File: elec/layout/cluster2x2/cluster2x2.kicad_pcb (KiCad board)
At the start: 2 copper layers, 20 parts

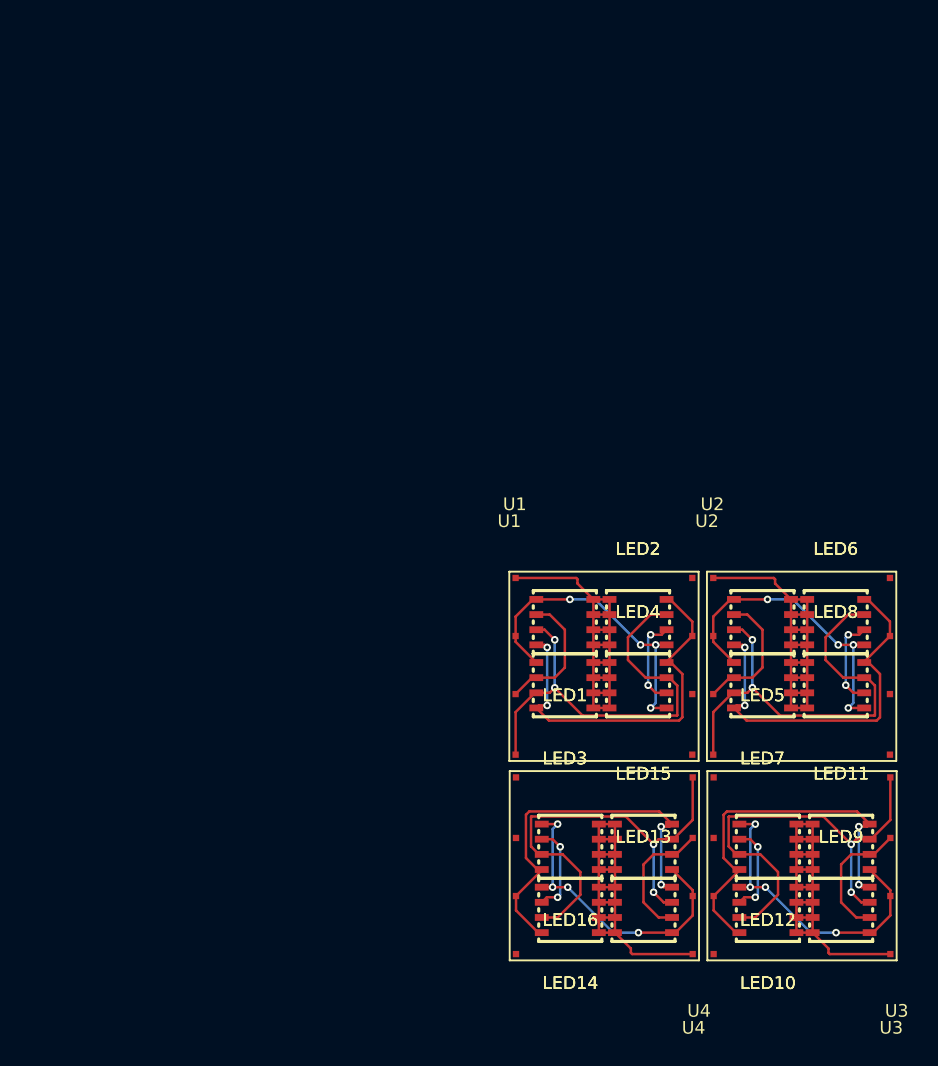
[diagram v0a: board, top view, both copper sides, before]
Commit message: cluster with driver
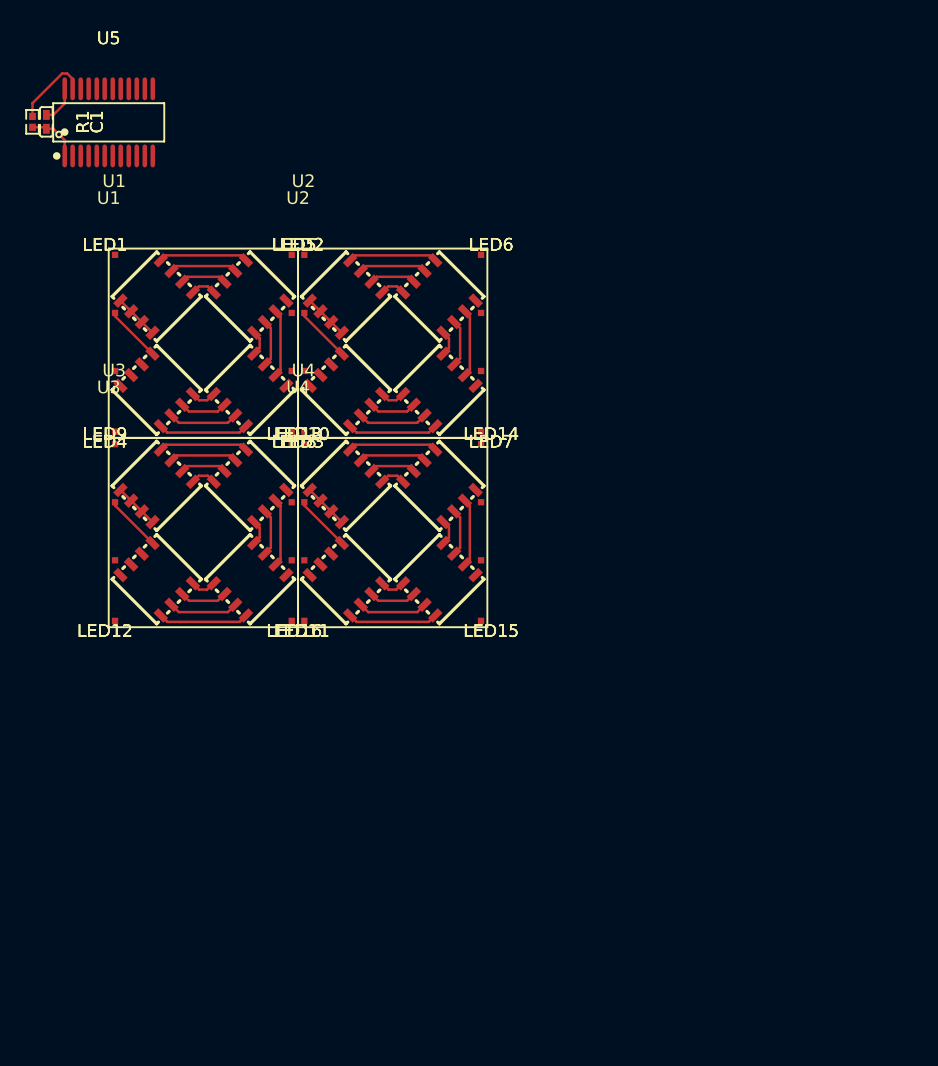
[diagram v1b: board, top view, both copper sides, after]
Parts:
- added C1: 100nF ±10% 16V X7R, Samsung_Electro_Mechanics_CL05B104KO5NNNC:C0402, F.Cu at (-4.94, -10.0)
- added R1: 309Ω ±1% 62.5mW, VO_SCR0402F309R:R0402, F.Cu at (-6.04, -10.0)
- added U5: , MBI_MBI5043GP_A:SSOP-24_L8.8-W4.0-P0.64-LS6.2-BL, F.Cu at (0.00, -10.0)
- moved U3 74.9 mm to (0.00, 15.0), turned to 0 degrees
- moved LED9 63.8 mm to (3.80, 18.8), turned to 45 degrees
- moved LED10 53.0 mm to (11.2, 18.8), turned to -45 degrees
- moved LED12 52.9 mm to (3.80, 26.2), turned to 135 degrees
- moved U4 52.2 mm to (15.0, 15.0), turned to 0 degrees
- moved LED11 51.4 mm to (11.2, 26.2), turned to -135 degrees
- moved LED8 45.3 mm to (18.8, 11.2), turned to 135 degrees
- moved LED4 44.7 mm to (3.80, 11.2), turned to 135 degrees
- moved LED5 41.9 mm to (18.8, 3.80), turned to 45 degrees
- moved LED1 41.4 mm to (3.80, 3.80), turned to 45 degrees
- moved U2 41.3 mm to (15.0, 0.00)
- moved LED13 41.0 mm to (18.8, 18.8), turned to 45 degrees
- moved U1 40.8 mm to (0.00, 0.00)
- moved LED6 40.6 mm to (26.2, 3.80), turned to -45 degrees
- moved LED2 40.1 mm to (11.2, 3.80), turned to -45 degrees
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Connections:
- net rows[0].pixels[0]-cathode_ir renamed rows[0].pixels[0]-ir
- net rows[0].pixels[0]-cathode_uv renamed rows[0].pixels[0]-uv
- net rows[0].pixels[0]-cathode_warm_white renamed rows[0].pixels[0]-warm_white
- net rows[0].pixels[1]-cathode_ir renamed rows[0].pixels[1]-ir
- net rows[0].pixels[1]-cathode_uv renamed rows[0].pixels[1]-uv
- net rows[0].pixels[1]-cathode_warm_white renamed rows[0].pixels[1]-warm_white
- net rows[1].pixels[0]-cathode_ir renamed rows[1].pixels[0]-ir
- net rows[1].pixels[0]-cathode_uv renamed rows[1].pixels[0]-uv
- net rows[1].pixels[0]-cathode_warm_white renamed rows[1].pixels[0]-warm_white
- net rows[1].pixels[1]-cathode_ir renamed rows[1].pixels[1]-ir
- net rows[1].pixels[1]-cathode_uv renamed rows[1].pixels[1]-uv
- net rows[1].pixels[1]-cathode_warm_white renamed rows[1].pixels[1]-warm_white
- LED1 pad 1: rows[0].pixels[0]-cathode_cold_white -> rows[0].pixels[0]-cold_white-1
- LED1 pad 2: rows[0].pixels[0]-anode -> -anode
- LED1 pad 3: rows[0].pixels[0]-cathode_blue -> rows[0].pixels[0]-blue-1
- LED1 pad 4: rows[0].pixels[0]-anode -> -anode
- LED1 pad 5: rows[0].pixels[0]-cathode_green -> rows[0].pixels[0]-green-1
- LED1 pad 6: rows[0].pixels[0]-anode -> -anode
- LED1 pad 7: rows[0].pixels[0]-cathode_red -> rows[0].pixels[0]-red-0
- LED1 pad 8: rows[0].pixels[0]-anode -> -anode
- LED10 pad 1: rows[1].pixels[0]-cathode_cold_white -> rows[1].pixels[0]-cold_white-2
- LED10 pad 2: rows[1].pixels[0]-anode -> rows[1].pixels[0]-cold_white-1
- LED10 pad 3: rows[1].pixels[0]-cathode_blue -> rows[1].pixels[0]-blue-2
- LED10 pad 4: rows[1].pixels[0]-anode -> rows[1].pixels[0]-blue-1
- LED10 pad 5: rows[1].pixels[0]-cathode_green -> rows[1].pixels[0]-green-2
- LED10 pad 6: rows[1].pixels[0]-anode -> rows[1].pixels[0]-green-1
- LED10 pad 7: rows[1].pixels[0]-cathode_red -> rows[1].pixels[0]-red-2
- LED10 pad 8: rows[1].pixels[0]-anode -> rows[1].pixels[0]-red-1
- LED11 pad 1: rows[1].pixels[0]-cathode_cold_white -> rows[1].pixels[0]-cold_white-3
- LED11 pad 2: rows[1].pixels[0]-anode -> rows[1].pixels[0]-cold_white-2
- LED11 pad 3: rows[1].pixels[0]-cathode_blue -> rows[1].pixels[0]-blue-3
- LED11 pad 4: rows[1].pixels[0]-anode -> rows[1].pixels[0]-blue-2
- LED11 pad 5: rows[1].pixels[0]-cathode_green -> rows[1].pixels[0]-green-3
- LED11 pad 6: rows[1].pixels[0]-anode -> rows[1].pixels[0]-green-2
- LED11 pad 7: rows[1].pixels[0]-cathode_red -> rows[1].pixels[0]-red-3
- LED11 pad 8: rows[1].pixels[0]-anode -> rows[1].pixels[0]-red-2
- LED12 pad 1: rows[1].pixels[0]-cathode_cold_white -> rows[1].pixels[0]-cold_white-0
- LED12 pad 2: rows[1].pixels[0]-anode -> rows[1].pixels[0]-cold_white-3
- LED12 pad 3: rows[1].pixels[0]-cathode_blue -> rows[1].pixels[0]-blue-0
- LED12 pad 4: rows[1].pixels[0]-anode -> rows[1].pixels[0]-blue-3
- LED12 pad 5: rows[1].pixels[0]-cathode_green -> rows[1].pixels[0]-green-0
- LED12 pad 6: rows[1].pixels[0]-anode -> rows[1].pixels[0]-green-3
- LED12 pad 7: rows[1].pixels[0]-cathode_red -> rows[1].pixels[0]-red-0
- LED12 pad 8: rows[1].pixels[0]-anode -> rows[1].pixels[0]-red-3
- LED13 pad 1: rows[1].pixels[1]-cathode_cold_white -> rows[1].pixels[1]-cold_white-1
- LED13 pad 3: rows[1].pixels[1]-cathode_blue -> rows[1].pixels[1]-blue-1
- LED13 pad 5: rows[1].pixels[1]-cathode_green -> rows[1].pixels[1]-green-1
- LED13 pad 7: rows[1].pixels[1]-cathode_red -> rows[1].pixels[1]-red-1
- LED14 pad 1: rows[1].pixels[1]-cathode_cold_white -> rows[1].pixels[1]-cold_white-2
- LED14 pad 2: rows[1].pixels[1]-anode -> rows[1].pixels[1]-cold_white-1
- LED14 pad 3: rows[1].pixels[1]-cathode_blue -> rows[1].pixels[1]-blue-2
- LED14 pad 4: rows[1].pixels[1]-anode -> rows[1].pixels[1]-blue-1
- LED14 pad 5: rows[1].pixels[1]-cathode_green -> rows[1].pixels[1]-green-2
- LED14 pad 6: rows[1].pixels[1]-anode -> rows[1].pixels[1]-green-1
- LED14 pad 7: rows[1].pixels[1]-cathode_red -> rows[1].pixels[1]-red-2
- LED14 pad 8: rows[1].pixels[1]-anode -> rows[1].pixels[1]-red-1
- LED15 pad 1: rows[1].pixels[1]-cathode_cold_white -> rows[1].pixels[1]-cold_white-3
- LED15 pad 2: rows[1].pixels[1]-anode -> rows[1].pixels[1]-cold_white-2
- LED15 pad 3: rows[1].pixels[1]-cathode_blue -> rows[1].pixels[1]-blue-3
- LED15 pad 4: rows[1].pixels[1]-anode -> rows[1].pixels[1]-blue-2
- LED15 pad 5: rows[1].pixels[1]-cathode_green -> rows[1].pixels[1]-green-3
- LED15 pad 6: rows[1].pixels[1]-anode -> rows[1].pixels[1]-green-2
- LED15 pad 7: rows[1].pixels[1]-cathode_red -> rows[1].pixels[1]-red-3
- LED15 pad 8: rows[1].pixels[1]-anode -> rows[1].pixels[1]-red-2
- LED16 pad 1: rows[1].pixels[1]-cathode_cold_white -> rows[1].pixels[1]-cold_white-0
- LED16 pad 2: rows[1].pixels[1]-anode -> rows[1].pixels[1]-cold_white-3
- LED16 pad 3: rows[1].pixels[1]-cathode_blue -> rows[1].pixels[1]-blue-0
- LED16 pad 4: rows[1].pixels[1]-anode -> rows[1].pixels[1]-blue-3
- LED16 pad 5: rows[1].pixels[1]-cathode_green -> rows[1].pixels[1]-green-0
- LED16 pad 6: rows[1].pixels[1]-anode -> rows[1].pixels[1]-green-3
- LED16 pad 7: rows[1].pixels[1]-cathode_red -> rows[1].pixels[1]-red-0
- LED16 pad 8: rows[1].pixels[1]-anode -> rows[1].pixels[1]-red-3
- LED2 pad 1: rows[0].pixels[0]-cathode_cold_white -> rows[0].pixels[0]-cold_white-2
- LED2 pad 2: rows[0].pixels[0]-anode -> rows[0].pixels[0]-cold_white-1
- LED2 pad 3: rows[0].pixels[0]-cathode_blue -> rows[0].pixels[0]-blue-2
- LED2 pad 4: rows[0].pixels[0]-anode -> rows[0].pixels[0]-blue-1
- LED2 pad 5: rows[0].pixels[0]-cathode_green -> rows[0].pixels[0]-green-2
- LED2 pad 6: rows[0].pixels[0]-anode -> rows[0].pixels[0]-green-1
- LED2 pad 7: rows[0].pixels[0]-cathode_red -> rows[0].pixels[0]-red-1
- LED2 pad 8: rows[0].pixels[0]-anode -> rows[0].pixels[0]-red-0
- LED3 pad 1: rows[0].pixels[0]-cathode_cold_white -> rows[0].pixels[0]-cold_white-3
- LED3 pad 2: rows[0].pixels[0]-anode -> rows[0].pixels[0]-cold_white-2
- LED3 pad 3: rows[0].pixels[0]-cathode_blue -> rows[0].pixels[0]-blue-3
- LED3 pad 4: rows[0].pixels[0]-anode -> rows[0].pixels[0]-blue-2
- LED3 pad 5: rows[0].pixels[0]-cathode_green -> rows[0].pixels[0]-green-3
- LED3 pad 6: rows[0].pixels[0]-anode -> rows[0].pixels[0]-green-2
- LED3 pad 7: rows[0].pixels[0]-cathode_red -> rows[0].pixels[0]-red-2
- LED3 pad 8: rows[0].pixels[0]-anode -> rows[0].pixels[0]-red-1
- LED4 pad 1: rows[0].pixels[0]-cathode_cold_white -> rows[0].pixels[0]-cold_white-0
- LED4 pad 2: rows[0].pixels[0]-anode -> rows[0].pixels[0]-cold_white-3
- LED4 pad 3: rows[0].pixels[0]-cathode_blue -> rows[0].pixels[0]-blue-0
- LED4 pad 4: rows[0].pixels[0]-anode -> rows[0].pixels[0]-blue-3
- LED4 pad 5: rows[0].pixels[0]-cathode_green -> rows[0].pixels[0]-green-0
- LED4 pad 6: rows[0].pixels[0]-anode -> rows[0].pixels[0]-green-3
- LED4 pad 7: rows[0].pixels[0]-cathode_red -> -red
- LED4 pad 8: rows[0].pixels[0]-anode -> rows[0].pixels[0]-red-2
- LED5 pad 1: rows[0].pixels[1]-cathode_cold_white -> rows[0].pixels[1]-cold_white-1
- LED5 pad 3: rows[0].pixels[1]-cathode_blue -> rows[0].pixels[1]-blue-1
- LED5 pad 5: rows[0].pixels[1]-cathode_green -> rows[0].pixels[1]-green-1
- LED5 pad 7: rows[0].pixels[1]-cathode_red -> rows[0].pixels[1]-red-1
- LED6 pad 1: rows[0].pixels[1]-cathode_cold_white -> rows[0].pixels[1]-cold_white-2
- LED6 pad 2: rows[0].pixels[1]-anode -> rows[0].pixels[1]-cold_white-1
- LED6 pad 3: rows[0].pixels[1]-cathode_blue -> rows[0].pixels[1]-blue-2
- LED6 pad 4: rows[0].pixels[1]-anode -> rows[0].pixels[1]-blue-1
- LED6 pad 5: rows[0].pixels[1]-cathode_green -> rows[0].pixels[1]-green-2
- LED6 pad 6: rows[0].pixels[1]-anode -> rows[0].pixels[1]-green-1
- LED6 pad 7: rows[0].pixels[1]-cathode_red -> rows[0].pixels[1]-red-2
- LED6 pad 8: rows[0].pixels[1]-anode -> rows[0].pixels[1]-red-1
- LED7 pad 1: rows[0].pixels[1]-cathode_cold_white -> rows[0].pixels[1]-cold_white-3
- LED7 pad 2: rows[0].pixels[1]-anode -> rows[0].pixels[1]-cold_white-2
- LED7 pad 3: rows[0].pixels[1]-cathode_blue -> rows[0].pixels[1]-blue-3
- LED7 pad 4: rows[0].pixels[1]-anode -> rows[0].pixels[1]-blue-2
- LED7 pad 5: rows[0].pixels[1]-cathode_green -> rows[0].pixels[1]-green-3
- LED7 pad 6: rows[0].pixels[1]-anode -> rows[0].pixels[1]-green-2
- LED7 pad 7: rows[0].pixels[1]-cathode_red -> rows[0].pixels[1]-red-3
- LED7 pad 8: rows[0].pixels[1]-anode -> rows[0].pixels[1]-red-2
- LED8 pad 1: rows[0].pixels[1]-cathode_cold_white -> rows[0].pixels[1]-cold_white-0
- LED8 pad 2: rows[0].pixels[1]-anode -> rows[0].pixels[1]-cold_white-3
- LED8 pad 3: rows[0].pixels[1]-cathode_blue -> rows[0].pixels[1]-blue-0
- LED8 pad 4: rows[0].pixels[1]-anode -> rows[0].pixels[1]-blue-3
- LED8 pad 5: rows[0].pixels[1]-cathode_green -> rows[0].pixels[1]-green-0
- LED8 pad 6: rows[0].pixels[1]-anode -> rows[0].pixels[1]-green-3
- LED8 pad 7: rows[0].pixels[1]-cathode_red -> rows[0].pixels[1]-red-0
- LED8 pad 8: rows[0].pixels[1]-anode -> rows[0].pixels[1]-red-3
- LED9 pad 1: rows[1].pixels[0]-cathode_cold_white -> rows[1].pixels[0]-cold_white-1
- LED9 pad 3: rows[1].pixels[0]-cathode_blue -> rows[1].pixels[0]-blue-1
- LED9 pad 5: rows[1].pixels[0]-cathode_green -> rows[1].pixels[0]-green-1
- LED9 pad 7: rows[1].pixels[0]-cathode_red -> rows[1].pixels[0]-red-1
- U1 pad 1: rows[0].pixels[0]-anode -> -anode
- U1 pad 2: rows[0].pixels[0]-cathode_red -> -red
- U1 pad 3: rows[0].pixels[0]-cathode_green -> rows[0].pixels[0]-green-0
- U1 pad 4: rows[0].pixels[0]-cathode_blue -> rows[0].pixels[0]-blue-0
- U1 pad 6: rows[0].pixels[0]-cathode_cold_white -> rows[0].pixels[0]-cold_white-0
- U2 pad 2: rows[0].pixels[1]-cathode_red -> rows[0].pixels[1]-red-0
- U2 pad 3: rows[0].pixels[1]-cathode_green -> rows[0].pixels[1]-green-0
- U2 pad 4: rows[0].pixels[1]-cathode_blue -> rows[0].pixels[1]-blue-0
- U2 pad 6: rows[0].pixels[1]-cathode_cold_white -> rows[0].pixels[1]-cold_white-0
- U3 pad 2: rows[1].pixels[0]-cathode_red -> rows[1].pixels[0]-red-0
- U3 pad 3: rows[1].pixels[0]-cathode_green -> rows[1].pixels[0]-green-0
- U3 pad 4: rows[1].pixels[0]-cathode_blue -> rows[1].pixels[0]-blue-0
- U3 pad 6: rows[1].pixels[0]-cathode_cold_white -> rows[1].pixels[0]-cold_white-0
- U4 pad 2: rows[1].pixels[1]-cathode_red -> rows[1].pixels[1]-red-0
- U4 pad 3: rows[1].pixels[1]-cathode_green -> rows[1].pixels[1]-green-0
- U4 pad 4: rows[1].pixels[1]-cathode_blue -> rows[1].pixels[1]-blue-0
- U4 pad 6: rows[1].pixels[1]-cathode_cold_white -> rows[1].pixels[1]-cold_white-0
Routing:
- net rows[1].pixels[0]-cathode_blue: track 36.2 -> 0.00 mm, vias 2 -> 0
- net rows[0].pixels[1]-cathode_blue: track 36.2 -> 0.00 mm, vias 2 -> 0
- net rows[1].pixels[1]-cathode_blue: track 36.2 -> 0.00 mm, vias 2 -> 0
- net rows[0].pixels[0]-cathode_blue: track 36.2 -> 0.00 mm, vias 2 -> 0
- net rows[0].pixels[0]-anode: track 34.5 -> 0.00 mm
- net rows[1].pixels[1]-anode: track 34.5 -> 3.60 mm
- net rows[0].pixels[1]-anode: track 34.5 -> 3.60 mm
- net rows[1].pixels[0]-anode: track 34.5 -> 3.60 mm
- net rows[0].pixels[0]-cathode_cold_white: track 30.5 -> 0.00 mm, vias 2 -> 0
- net rows[1].pixels[1]-cathode_cold_white: track 30.5 -> 0.00 mm, vias 2 -> 0
- net rows[0].pixels[1]-cathode_cold_white: track 30.5 -> 0.00 mm, vias 2 -> 0
- net rows[1].pixels[0]-cathode_cold_white: track 30.5 -> 0.00 mm, vias 2 -> 0
- net rows[0].pixels[1]-cathode_red: track 24.8 -> 0.00 mm, vias 4 -> 0
- net rows[1].pixels[0]-cathode_red: track 24.8 -> 0.00 mm, vias 4 -> 0
- net rows[0].pixels[0]-cathode_red: track 24.8 -> 0.00 mm, vias 4 -> 0
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
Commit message: broken kicad file
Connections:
- net -red renamed -red-0
- LED1 pad 1: rows[0].pixels[0]-cold_white-1 -> rows[0].pixels[0]-cold_white-0
- LED1 pad 2: -anode -> anode
- LED1 pad 3: rows[0].pixels[0]-blue-1 -> rows[0].pixels[0]-blue-0
- LED1 pad 4: -anode -> anode
- LED1 pad 5: rows[0].pixels[0]-green-1 -> rows[0].pixels[0]-green-0
- LED1 pad 6: -anode -> anode
- LED1 pad 8: -anode -> anode
- LED10 pad 1: rows[1].pixels[0]-cold_white-2 -> rows[1].pixels[0]-cold_white-1
- LED10 pad 2: rows[1].pixels[0]-cold_white-1 -> rows[1].pixels[0]-cold_white-0
- LED10 pad 3: rows[1].pixels[0]-blue-2 -> rows[1].pixels[0]-blue-1
- LED10 pad 4: rows[1].pixels[0]-blue-1 -> rows[1].pixels[0]-blue-0
- LED10 pad 5: rows[1].pixels[0]-green-2 -> rows[1].pixels[0]-green-1
- LED10 pad 6: rows[1].pixels[0]-green-1 -> rows[1].pixels[0]-green-0
- LED10 pad 7: rows[1].pixels[0]-red-2 -> rows[1].pixels[0]-red-1
- LED10 pad 8: rows[1].pixels[0]-red-1 -> rows[1].pixels[0]-red-0
- LED11 pad 1: rows[1].pixels[0]-cold_white-3 -> rows[1].pixels[0]-cold_white-2
- LED11 pad 2: rows[1].pixels[0]-cold_white-2 -> rows[1].pixels[0]-cold_white-1
- LED11 pad 3: rows[1].pixels[0]-blue-3 -> rows[1].pixels[0]-blue-2
- LED11 pad 4: rows[1].pixels[0]-blue-2 -> rows[1].pixels[0]-blue-1
- LED11 pad 5: rows[1].pixels[0]-green-3 -> rows[1].pixels[0]-green-2
- LED11 pad 6: rows[1].pixels[0]-green-2 -> rows[1].pixels[0]-green-1
- LED11 pad 7: rows[1].pixels[0]-red-3 -> rows[1].pixels[0]-red-2
- LED11 pad 8: rows[1].pixels[0]-red-2 -> rows[1].pixels[0]-red-1
- LED12 pad 1: rows[1].pixels[0]-cold_white-0 -> -cold_white-0
- LED12 pad 2: rows[1].pixels[0]-cold_white-3 -> rows[1].pixels[0]-cold_white-2
- LED12 pad 3: rows[1].pixels[0]-blue-0 -> -blue-0
- LED12 pad 4: rows[1].pixels[0]-blue-3 -> rows[1].pixels[0]-blue-2
- LED12 pad 5: rows[1].pixels[0]-green-0 -> -green-3
- LED12 pad 6: rows[1].pixels[0]-green-3 -> rows[1].pixels[0]-green-2
- LED12 pad 7: rows[1].pixels[0]-red-0 -> -red-3
- LED12 pad 8: rows[1].pixels[0]-red-3 -> rows[1].pixels[0]-red-2
- LED13 pad 1: rows[1].pixels[1]-cold_white-1 -> rows[1].pixels[1]-cold_white-0
- LED13 pad 2: rows[1].pixels[1]-anode -> anode
- LED13 pad 3: rows[1].pixels[1]-blue-1 -> rows[1].pixels[1]-blue-0
- LED13 pad 4: rows[1].pixels[1]-anode -> anode
- LED13 pad 5: rows[1].pixels[1]-green-1 -> rows[1].pixels[1]-green-0
- LED13 pad 6: rows[1].pixels[1]-anode -> anode
- LED13 pad 7: rows[1].pixels[1]-red-1 -> rows[1].pixels[1]-red-0
- LED13 pad 8: rows[1].pixels[1]-anode -> anode
- LED14 pad 1: rows[1].pixels[1]-cold_white-2 -> rows[1].pixels[1]-cold_white-1
- LED14 pad 2: rows[1].pixels[1]-cold_white-1 -> rows[1].pixels[1]-cold_white-0
- LED14 pad 3: rows[1].pixels[1]-blue-2 -> rows[1].pixels[1]-blue-1
- LED14 pad 4: rows[1].pixels[1]-blue-1 -> rows[1].pixels[1]-blue-0
- LED14 pad 5: rows[1].pixels[1]-green-2 -> rows[1].pixels[1]-green-1
- LED14 pad 6: rows[1].pixels[1]-green-1 -> rows[1].pixels[1]-green-0
- LED14 pad 7: rows[1].pixels[1]-red-2 -> rows[1].pixels[1]-red-1
- LED14 pad 8: rows[1].pixels[1]-red-1 -> rows[1].pixels[1]-red-0
- LED15 pad 1: rows[1].pixels[1]-cold_white-3 -> rows[1].pixels[1]-cold_white-2
- LED15 pad 2: rows[1].pixels[1]-cold_white-2 -> rows[1].pixels[1]-cold_white-1
- LED15 pad 3: rows[1].pixels[1]-blue-3 -> rows[1].pixels[1]-blue-2
- LED15 pad 4: rows[1].pixels[1]-blue-2 -> rows[1].pixels[1]-blue-1
- LED15 pad 5: rows[1].pixels[1]-green-3 -> rows[1].pixels[1]-green-2
- LED15 pad 6: rows[1].pixels[1]-green-2 -> rows[1].pixels[1]-green-1
- LED15 pad 7: rows[1].pixels[1]-red-3 -> rows[1].pixels[1]-red-2
- LED15 pad 8: rows[1].pixels[1]-red-2 -> rows[1].pixels[1]-red-1
- LED16 pad 1: rows[1].pixels[1]-cold_white-0 -> -cold_white-1
- LED16 pad 2: rows[1].pixels[1]-cold_white-3 -> rows[1].pixels[1]-cold_white-2
- LED16 pad 3: rows[1].pixels[1]-blue-0 -> -blue-1
- LED16 pad 4: rows[1].pixels[1]-blue-3 -> rows[1].pixels[1]-blue-2
- LED16 pad 5: rows[1].pixels[1]-green-0 -> -green-0
- LED16 pad 6: rows[1].pixels[1]-green-3 -> rows[1].pixels[1]-green-2
- LED16 pad 7: rows[1].pixels[1]-red-0 -> -red-1
- LED16 pad 8: rows[1].pixels[1]-red-3 -> rows[1].pixels[1]-red-2
- LED2 pad 1: rows[0].pixels[0]-cold_white-2 -> rows[0].pixels[0]-cold_white-1
- LED2 pad 2: rows[0].pixels[0]-cold_white-1 -> rows[0].pixels[0]-cold_white-0
- LED2 pad 3: rows[0].pixels[0]-blue-2 -> rows[0].pixels[0]-blue-1
- LED2 pad 4: rows[0].pixels[0]-blue-1 -> rows[0].pixels[0]-blue-0
- LED2 pad 5: rows[0].pixels[0]-green-2 -> rows[0].pixels[0]-green-1
- LED2 pad 6: rows[0].pixels[0]-green-1 -> rows[0].pixels[0]-green-0
- LED3 pad 1: rows[0].pixels[0]-cold_white-3 -> rows[0].pixels[0]-cold_white-2
- LED3 pad 2: rows[0].pixels[0]-cold_white-2 -> rows[0].pixels[0]-cold_white-1
- LED3 pad 3: rows[0].pixels[0]-blue-3 -> rows[0].pixels[0]-blue-2
- LED3 pad 4: rows[0].pixels[0]-blue-2 -> rows[0].pixels[0]-blue-1
- LED3 pad 5: rows[0].pixels[0]-green-3 -> rows[0].pixels[0]-green-2
- LED3 pad 6: rows[0].pixels[0]-green-2 -> rows[0].pixels[0]-green-1
- LED4 pad 1: rows[0].pixels[0]-cold_white-0 -> -cold_white-2
- LED4 pad 2: rows[0].pixels[0]-cold_white-3 -> rows[0].pixels[0]-cold_white-2
- LED4 pad 3: rows[0].pixels[0]-blue-0 -> -blue-2
- LED4 pad 4: rows[0].pixels[0]-blue-3 -> rows[0].pixels[0]-blue-2
- LED4 pad 5: rows[0].pixels[0]-green-0 -> -green-1
- LED4 pad 6: rows[0].pixels[0]-green-3 -> rows[0].pixels[0]-green-2
- LED5 pad 1: rows[0].pixels[1]-cold_white-1 -> rows[0].pixels[1]-cold_white-0
- LED5 pad 2: rows[0].pixels[1]-anode -> anode
- LED5 pad 3: rows[0].pixels[1]-blue-1 -> rows[0].pixels[1]-blue-0
- LED5 pad 4: rows[0].pixels[1]-anode -> anode
- LED5 pad 5: rows[0].pixels[1]-green-1 -> rows[0].pixels[1]-green-0
- LED5 pad 6: rows[0].pixels[1]-anode -> anode
- LED5 pad 7: rows[0].pixels[1]-red-1 -> rows[0].pixels[1]-red-0
- LED5 pad 8: rows[0].pixels[1]-anode -> anode
- LED6 pad 1: rows[0].pixels[1]-cold_white-2 -> rows[0].pixels[1]-cold_white-1
- LED6 pad 2: rows[0].pixels[1]-cold_white-1 -> rows[0].pixels[1]-cold_white-0
- LED6 pad 3: rows[0].pixels[1]-blue-2 -> rows[0].pixels[1]-blue-1
- LED6 pad 4: rows[0].pixels[1]-blue-1 -> rows[0].pixels[1]-blue-0
- LED6 pad 5: rows[0].pixels[1]-green-2 -> rows[0].pixels[1]-green-1
- LED6 pad 6: rows[0].pixels[1]-green-1 -> rows[0].pixels[1]-green-0
- LED6 pad 7: rows[0].pixels[1]-red-2 -> rows[0].pixels[1]-red-1
- LED6 pad 8: rows[0].pixels[1]-red-1 -> rows[0].pixels[1]-red-0
- LED7 pad 1: rows[0].pixels[1]-cold_white-3 -> rows[0].pixels[1]-cold_white-2
- LED7 pad 2: rows[0].pixels[1]-cold_white-2 -> rows[0].pixels[1]-cold_white-1
- LED7 pad 3: rows[0].pixels[1]-blue-3 -> rows[0].pixels[1]-blue-2
- LED7 pad 4: rows[0].pixels[1]-blue-2 -> rows[0].pixels[1]-blue-1
- LED7 pad 5: rows[0].pixels[1]-green-3 -> rows[0].pixels[1]-green-2
- LED7 pad 6: rows[0].pixels[1]-green-2 -> rows[0].pixels[1]-green-1
- LED7 pad 7: rows[0].pixels[1]-red-3 -> rows[0].pixels[1]-red-2
- LED7 pad 8: rows[0].pixels[1]-red-2 -> rows[0].pixels[1]-red-1
- LED8 pad 1: rows[0].pixels[1]-cold_white-0 -> -cold_white-3
- LED8 pad 2: rows[0].pixels[1]-cold_white-3 -> rows[0].pixels[1]-cold_white-2
- LED8 pad 3: rows[0].pixels[1]-blue-0 -> -blue-3
- LED8 pad 4: rows[0].pixels[1]-blue-3 -> rows[0].pixels[1]-blue-2
- LED8 pad 5: rows[0].pixels[1]-green-0 -> -green-2
- LED8 pad 6: rows[0].pixels[1]-green-3 -> rows[0].pixels[1]-green-2
- LED8 pad 7: rows[0].pixels[1]-red-0 -> -red-2
- LED8 pad 8: rows[0].pixels[1]-red-3 -> rows[0].pixels[1]-red-2
- LED9 pad 1: rows[1].pixels[0]-cold_white-1 -> rows[1].pixels[0]-cold_white-0
- LED9 pad 2: rows[1].pixels[0]-anode -> anode
- LED9 pad 3: rows[1].pixels[0]-blue-1 -> rows[1].pixels[0]-blue-0
- LED9 pad 4: rows[1].pixels[0]-anode -> anode
- LED9 pad 5: rows[1].pixels[0]-green-1 -> rows[1].pixels[0]-green-0
- LED9 pad 6: rows[1].pixels[0]-anode -> anode
- LED9 pad 7: rows[1].pixels[0]-red-1 -> rows[1].pixels[0]-red-0
- LED9 pad 8: rows[1].pixels[0]-anode -> anode
- U1 pad 1: -anode -> anode
- U1 pad 3: rows[0].pixels[0]-green-0 -> -green-1
- U1 pad 4: rows[0].pixels[0]-blue-0 -> -blue-2
- U1 pad 6: rows[0].pixels[0]-cold_white-0 -> -cold_white-2
- U2 pad 1: rows[0].pixels[1]-anode -> anode
- U2 pad 2: rows[0].pixels[1]-red-0 -> -red-2
- U2 pad 3: rows[0].pixels[1]-green-0 -> -green-2
- U2 pad 4: rows[0].pixels[1]-blue-0 -> -blue-3
- U2 pad 6: rows[0].pixels[1]-cold_white-0 -> -cold_white-3
- U3 pad 1: rows[1].pixels[0]-anode -> anode
- U3 pad 2: rows[1].pixels[0]-red-0 -> -red-3
- U3 pad 3: rows[1].pixels[0]-green-0 -> -green-3
- U3 pad 4: rows[1].pixels[0]-blue-0 -> -blue-0
- U3 pad 6: rows[1].pixels[0]-cold_white-0 -> -cold_white-0
- U4 pad 1: rows[1].pixels[1]-anode -> anode
- U4 pad 2: rows[1].pixels[1]-red-0 -> -red-1
- U4 pad 3: rows[1].pixels[1]-green-0 -> -green-0
- U4 pad 4: rows[1].pixels[1]-blue-0 -> -blue-1
- U4 pad 6: rows[1].pixels[1]-cold_white-0 -> -cold_white-1
- U5 pad 10: OUT5 -> -green-2
- U5 pad 11: OUT6 -> -blue-3
- U5 pad 12: OUT7 -> -cold_white-3
- U5 pad 13: OUT8 -> -red-3
- U5 pad 14: OUT9 -> -green-3
- U5 pad 15: OUT10 -> -blue-0
- U5 pad 16: OUT11 -> -cold_white-0
- U5 pad 17: OUT12 -> -red-1
- U5 pad 18: OUT13 -> -green-0
- U5 pad 19: OUT14 -> -blue-1
- U5 pad 20: OUT15 -> -cold_white-1
- U5 pad 6: OUT1 -> -green-1
- U5 pad 7: OUT2 -> -blue-2
- U5 pad 8: OUT3 -> -cold_white-2
- U5 pad 9: OUT4 -> -red-2
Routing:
- net (no net): track 0.00 -> 27.8 mm
- net rows[1].pixels[1]-cold_white-3: track 7.17 -> 0.00 mm
- net rows[1].pixels[1]-cold_white-2: track 0.00 -> 7.17 mm
- net rows[0].pixels[1]-cold_white-3: track 7.17 -> 0.00 mm
- net rows[0].pixels[1]-cold_white-2: track 0.00 -> 7.17 mm
- net rows[1].pixels[0]-cold_white-3: track 7.17 -> 0.00 mm
- net rows[1].pixels[0]-cold_white-2: track 0.00 -> 7.17 mm
- net rows[0].pixels[0]-cold_white-3: track 7.17 -> 0.00 mm
- net rows[0].pixels[0]-cold_white-2: track 0.00 -> 7.17 mm
- net rows[1].pixels[1]-cold_white-1: track 7.07 -> 0.00 mm
- net rows[1].pixels[1]-cold_white-0: track 0.00 -> 7.07 mm
- net rows[1].pixels[0]-cold_white-1: track 7.07 -> 0.00 mm
- net rows[0].pixels[1]-cold_white-1: track 7.07 -> 0.00 mm
- net rows[0].pixels[1]-cold_white-0: track 0.00 -> 7.07 mm
- net rows[0].pixels[0]-cold_white-1: track 7.07 -> 0.00 mm
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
